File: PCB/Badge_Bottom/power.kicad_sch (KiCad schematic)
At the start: 10 parts, among them J2 BAT, SW3 MSK12C02-HB, U1 TP4054, U3 AMS1117-3.3

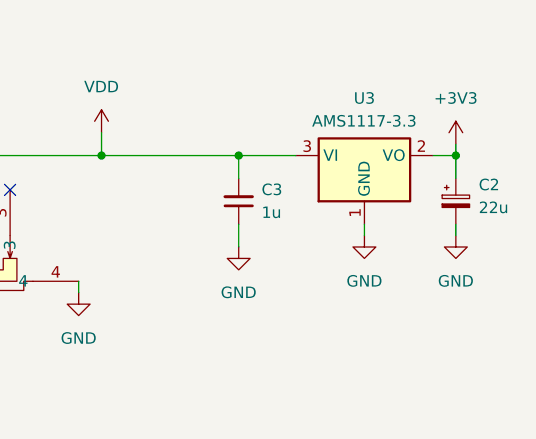
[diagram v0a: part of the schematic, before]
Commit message: finished schematic and added jlc parts
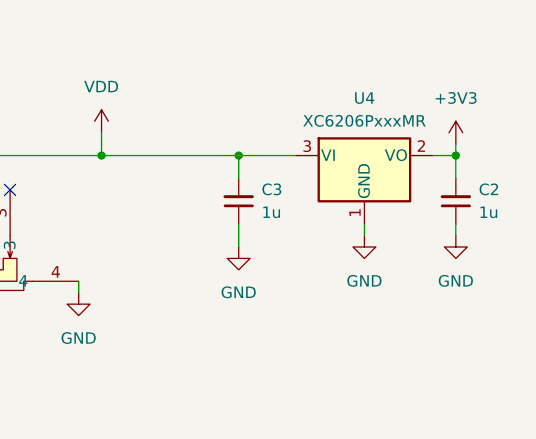
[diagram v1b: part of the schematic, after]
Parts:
- removed C2: 22u, Capacitor_SMD:C_0603_1608Metric, symbol Device:C_Polarized_Small
- removed U3: AMS1117-3.3, Package_TO_SOT_SMD:SOT-223-3_TabPin2, symbol Regulator_Linear:AMS1117-3.3
- added C2: 1u, Capacitor_SMD:C_0603_1608Metric, symbol Device:C_Small
- added U4: XC6206PxxxMR, Package_TO_SOT_SMD:SOT-23-3, symbol Regulator_Linear:XC6206PxxxMR
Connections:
- net +3V3: now also C2.2, U4.2 (VO)
- net GND: now also C2.1, U4.1 (GND)
- net VDD: now also U4.3 (VI)
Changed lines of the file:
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@@
+    )
+  )
+  (symbol (lib_id "Regulator_Linear:XC6206PxxxMR") (at 187.96 96.52 0) (unit 1)
+    (in_bom yes) (on_board yes) (dnp no) (fields_autoplaced)
+    (property "Reference" "U4" (at 187.96 90.17 0)
+      (effects (font (size 1.27 1.27)))
+    )
+    (property "Value" "XC6206PxxxMR" (at 187.96 92.71 0)
+      (effects (font (size 1.27 1.27)))
+    )
+    (property "Footprint" "Package_TO_SOT_SMD:SOT-23-3" (at 187.96 90.805 0)
+      (effects (font (size 1.27 1.27) italic) hide)
+    )
+    (property "Datasheet" "https://www.torexsemi.com/file/xc6206/XC6206.pdf" (at 187.96 96.52 0)
+      (effects (font (size 1.27 1.27)) hide)
+    )
+    (pin "1")
+    (pin "2")
+    (pin "3")
+    (instances
+      (project "Badge_Bottom"
+        (path "/9bea0129-61af-4534-9a88-a88b63234707/0f55777b-99bc-476f-91c2-8f0549bc7bba"
+          (reference "U4") (unit 1)
+        )
+      )
     )
   )
@@
     )
   )
-  (symbol (lib_id "Device:C_Polarized_Small") (at 198.12 101.6 0) (unit 1)
-    (in_bom yes) (on_board yes) (dnp no) (fields_autoplaced)
-    (property "Reference" "C2" (at 200.66 99.7839 0)
-      (effects (font (size 1.27 1.27)) (justify left))
-    )
-    (property "Value" "22u" (at 200.66 102.3239 0)
-      (effects (font (size 1.27 1.27)) (justify left))
-    )
-    (property "Footprint" "Capacitor_SMD:C_0603_1608Metric" (at 198.12 101.6 0)
-      (effects (font (size 1.27 1.27)) hide)
-    )
-    (property "Datasheet" "~" (at 198.12 101.6 0)
-      (effects (font (size 1.27 1.27)) hide)
-    )
-    (pin "1")
-    (pin "2")
-    (instances
-      (project "Badge_Bottom"
-        (path "/9bea0129-61af-4534-9a88-a88b63234707/0f55777b-99bc-476f-91c2-8f0549bc7bba"
-          (reference "C2") (unit 1)
-        )
-      )
-    )
-  )
   (symbol (lib_id "Device:LED") (at 82.55 99.06 180) (unit 1)
     (in_bom yes) (on_board yes) (dnp no) (fields_autoplaced)
@@
         (path "/9bea0129-61af-4534-9a88-a88b63234707/0f55777b-99bc-476f-91c2-8f0549bc7bba"
           (reference "D1") (unit 1)
-        )
-      )
-    )
-  )
-  (symbol (lib_id "Regulator_Linear:AMS1117-3.3") (at 187.96 96.52 0) (unit 1)
-    (in_bom yes) (on_board yes) (dnp no) (fields_autoplaced)
-    (property "Reference" "U3" (at 187.96 90.17 0)
-      (effects (font (size 1.27 1.27)))
-    )
-    (property "Value" "AMS1117-3.3" (at 187.96 92.71 0)
-      (effects (font (size 1.27 1.27)))
-    )
-    (property "Footprint" "Package_TO_SOT_SMD:SOT-223-3_TabPin2" (at 187.96 91.44 0)
-      (effects (font (size 1.27 1.27)) hide)
-    )
-    (property "Datasheet" "http://www.advanced-monolithic.com/pdf/ds1117.pdf" (at 190.5 102.87 0)
-      (effects (font (size 1.27 1.27)) hide)
-    )
-    (pin "1")
-    (pin "2")
-    (pin "3")
-    (instances
-      (project "Badge_Bottom"
-        (path "/9bea0129-61af-4534-9a88-a88b63234707/0f55777b-99bc-476f-91c2-8f0549bc7bba"
-          (reference "U3") (unit 1)
         )
       )
@@
         )
       )
+    )
+  )
+  (symbol (lib_id "Device:C_Small") (at 198.12 101.6 180) (unit 1)
+    (in_bom yes) (on_board yes) (dnp no) (fields_autoplaced)
+    (property "Reference" "C2" (at 200.66 100.3236 0)
+      (effects (font (size 1.27 1.27)) (justify right))
+    )
+    (property "Value" "1u" (at 200.66 102.8636 0)
+      (effects (font (size 1.27 1.27)) (justify right))
+    )
+    (property "Footprint" "Capacitor_SMD:C_0603_1608Metric" (at 198.12 101.6 0)
+      (effects (font (size 1.27 1.27)) hide)
+    )
+    (property "Datasheet" "~" (at 198.12 101.6 0)
+      (effects (font (size 1.27 1.27)) hide)
+    )
+    (pin "1")
+    (pin "2")
+    (instances
+      (project "Badge_Bottom"
+        (path "/9bea0129-61af-4534-9a88-a88b63234707/0f55777b-99bc-476f-91c2-8f0549bc7bba"
+          (reference "C2") (unit 1)
+        )
+      )

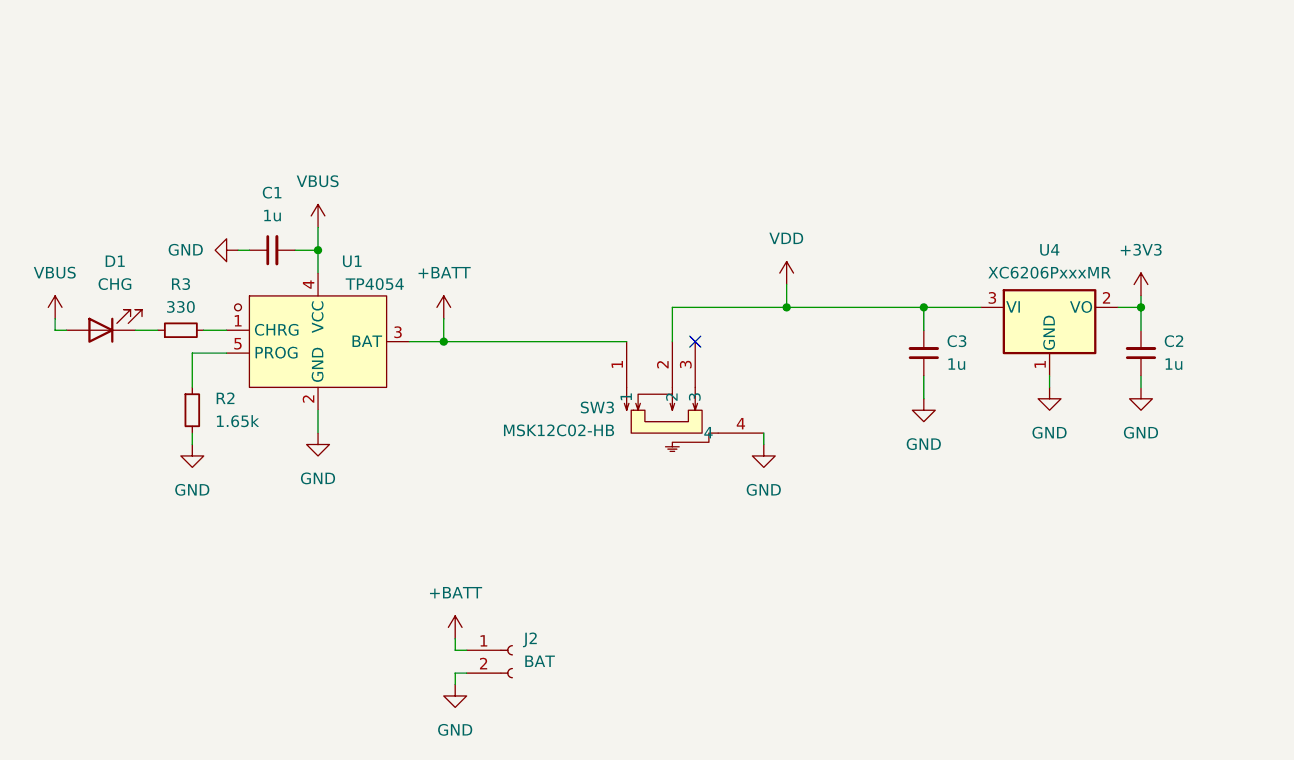
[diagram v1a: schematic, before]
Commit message: finised pcb layout
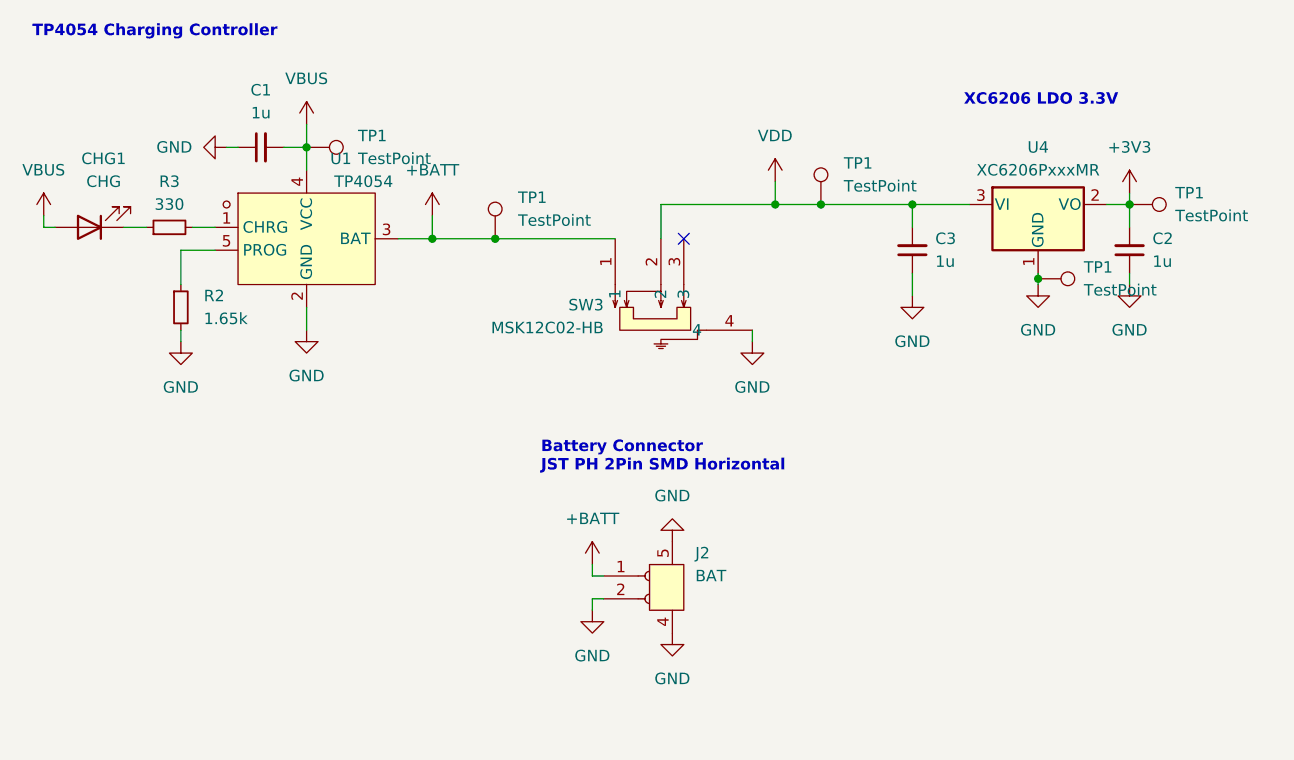
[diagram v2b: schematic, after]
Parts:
- added TP1 (x5): TestPoint, TestPoint:TestPoint_Pad_D1.0mm, symbol Connector:TestPoint
- J2: footprint Connector_JST:JST_PH_S2B-PH-SM4-TB_1x02-1MP_P2.00mm_Horizontal -> JSTPH_Clone:CONN-SMD_2P-P2.00_XUNPU_WAFER-PH2.0-2PWB
- renumbered D1 to CHG1
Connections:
- net +3V3: now also TP1.1
- net +BATT: now also TP1.1
- net GND: now also J2.4 (MP), J2.5 (MP), TP1.1
- net VBUS: now also TP1.1
- net VDD: now also TP1.1
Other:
- note added: "Battery Connector JST PH 2Pin SMD Horizontal"
- note added: "TP4054 Charging Controller"
- note added: "XC6206 LDO 3.3V"
- moved on the sheet: C1, C2, C3, CHG1, R2, R3, SW3, U1, U4

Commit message: Added docs and readme, ordered PCBs at JLC
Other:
- company: (none) -> Unterland
- title: (none) -> Unterland Badge Bottom
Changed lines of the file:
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@@
 (kicad_sch (version 20230121) (generator eeschema)
   (paper "A4")
+  (title_block
+    (title "Unterland Badge Bottom")
+    (date "2023-07-29")
+    (rev "1")
+    (company "Unterland")
+    (comment 1 "Power Section")
+  )
   (junction (at 172.72 85.09) (diameter 0) (color 0 0 0 0)
   )
